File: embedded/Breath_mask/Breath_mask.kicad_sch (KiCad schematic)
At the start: 33 parts, among them IC1 TPS61291DRVR, J1 Conn_01x02_Pin, J2 USB, J4 Conn_ST_STDC14, SW2 SW_Push, SW3 SW_Push, U1 LPS22HBTR, U23 M95256, U4 STM32L052K8Tx

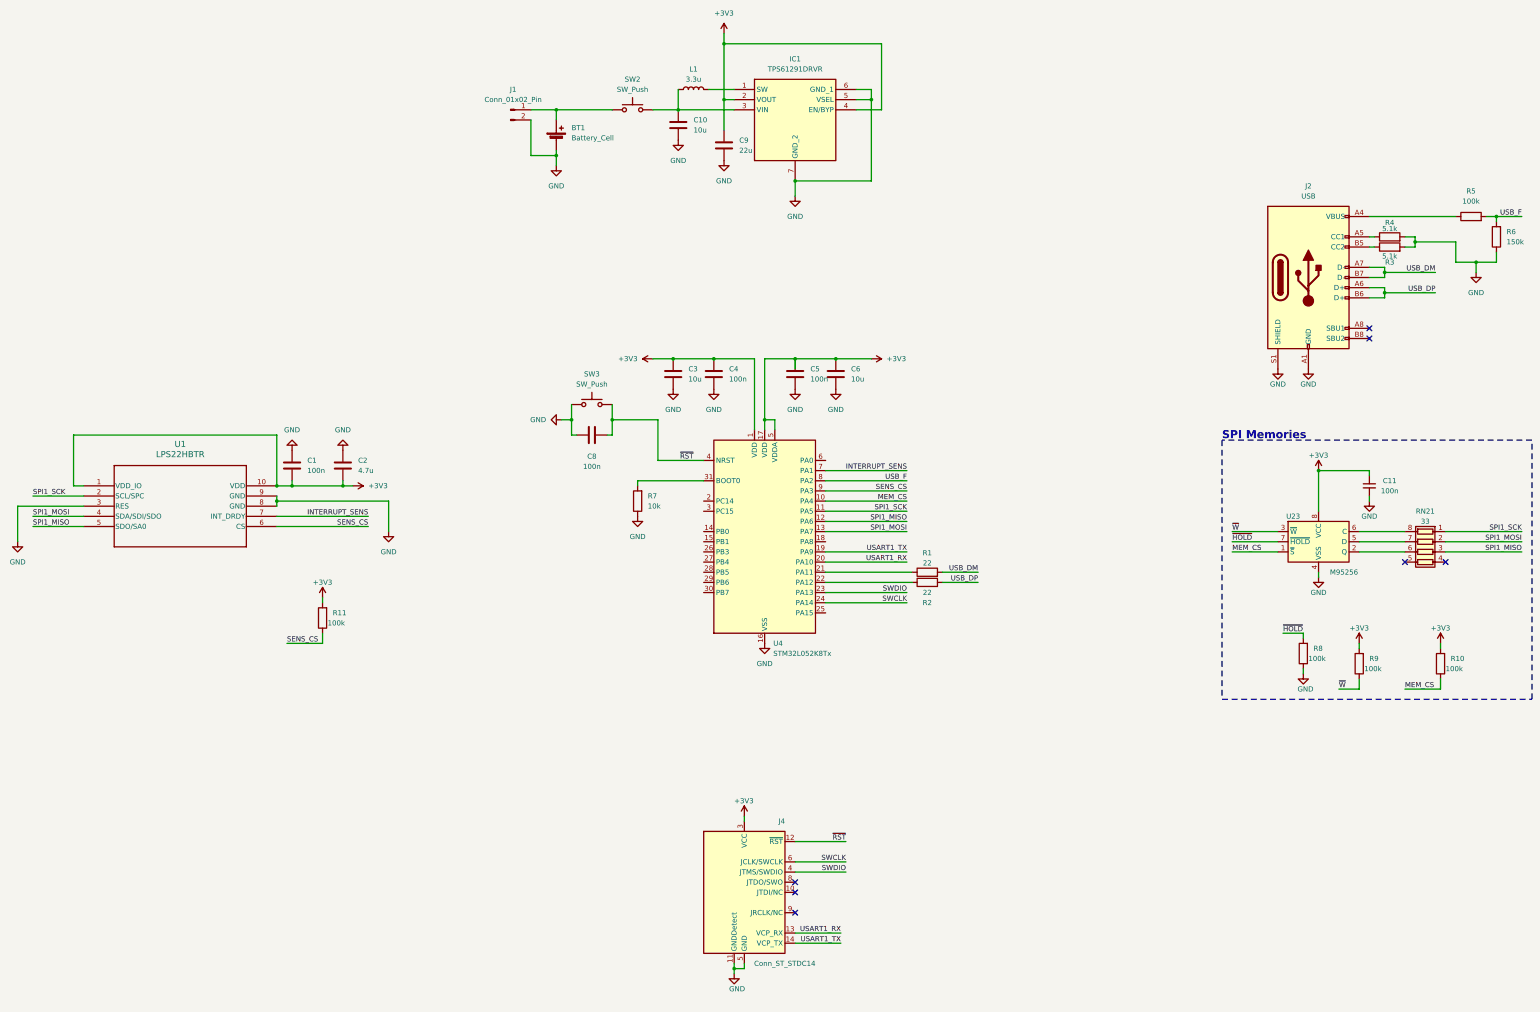
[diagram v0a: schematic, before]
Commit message: inizio sbroglio pcb
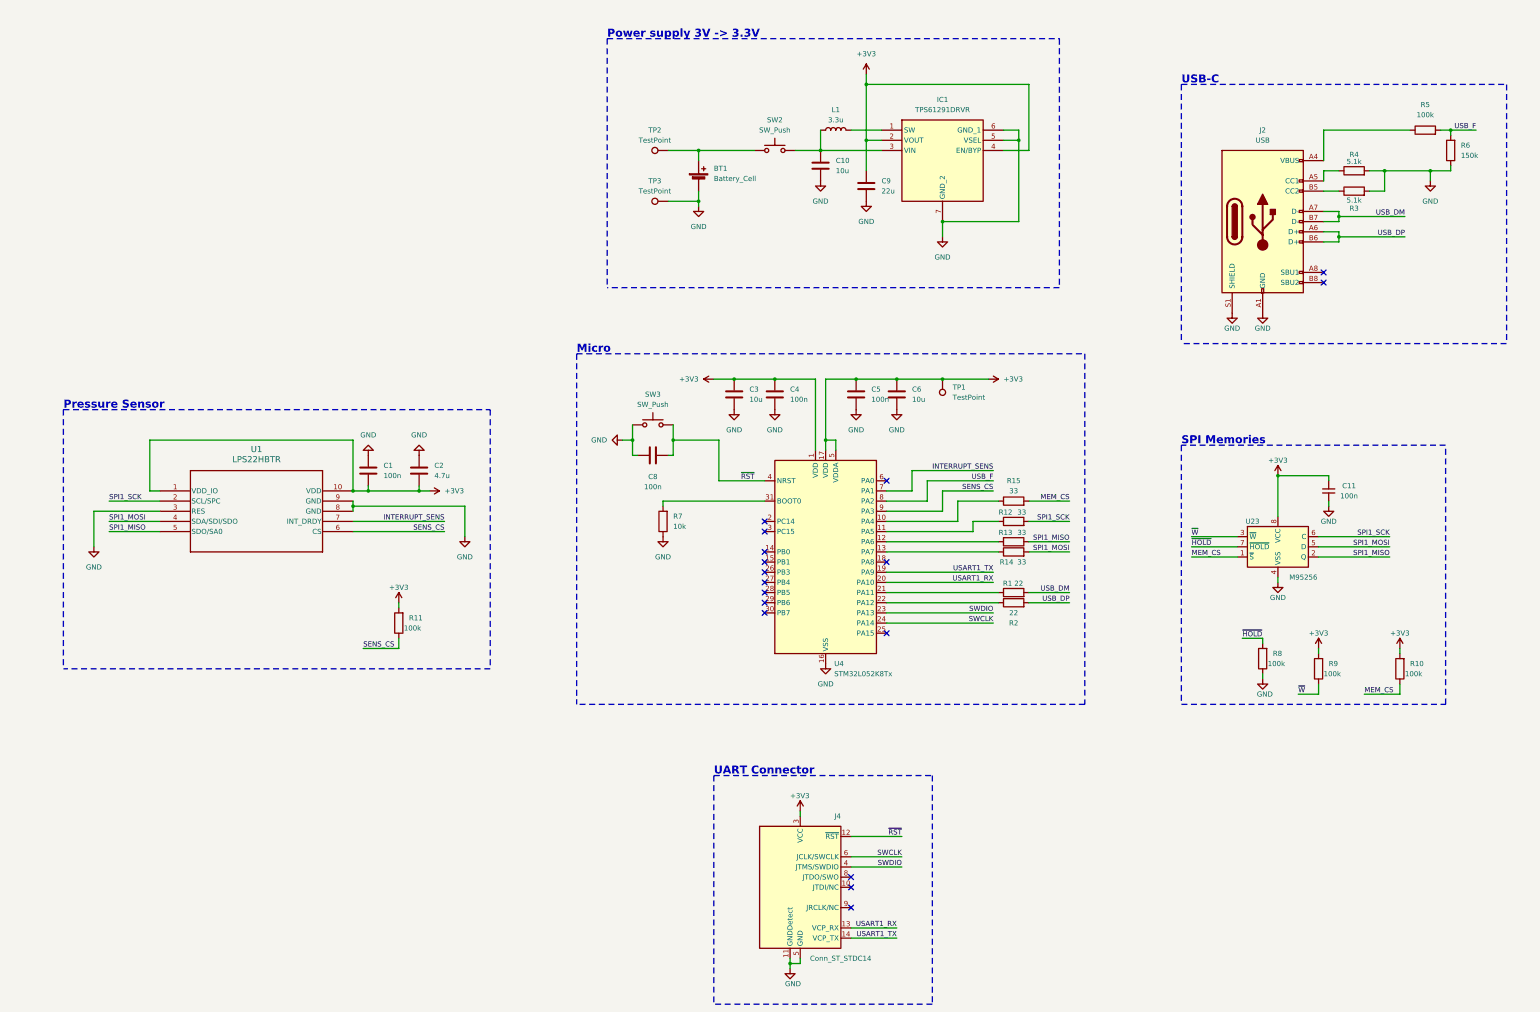
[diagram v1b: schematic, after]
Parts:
- removed J1: Conn_01x02_Pin, symbol Connector:Conn_01x02_Pin
- removed RN21: 33, Resistor_SMD:R_Array_Convex_4x0603, symbol Device:R_Pack04
- added R12, R13, R14, R15: 33, Resistor_SMD:R_0603_1608Metric, symbol Device:R
- added TP1, TP2, TP3: TestPoint, TestPoint:TestPoint_Pad_D1.0mm, symbol Connector:TestPoint
- BT1: footprint (none) -> Battery:BatteryHolder_Keystone_3034_1x20mm
- C1, C2, C4, C5, C8: footprint (none) -> Capacitor_SMD:C_0603_1608Metric
- C10, C3, C6, C9: footprint (none) -> Capacitor_SMD:C_0805_2012Metric
- IC1: footprint SON65P200X200X80-7N -> Package_SON:WSON-6-1EP_2x2mm_P0.65mm_EP1x1.6mm_ThermalVias
- J4: footprint eagle_connectors:SAMTEC_FTSH-107-01-L-DV-K-TR -> impronte_breath_mask:SAMTEC_FTSH-107-01-L-DV-K-TR
- L1: footprint (none) -> Inductor_SMD:L_Coilcraft_LPS3314
- R1, R2, R3, R4, R5, R6, R7: footprint (none) -> Resistor_SMD:R_0603_1608Metric
- SW2: footprint (none) -> Button_Switch_SMD:SW_SPDT_CK_JS102011SAQN
- SW3: footprint (none) -> Button_Switch_SMD:SW_Push_1P1T_XKB_TS-1187A
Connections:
- net +3V3: now also TP1.1
- net GND: now also TP3.1
- net MEM_CS: now also R15.2; no longer U4.10 (PA4)
- net SPI1_MISO: now also U23.2 (Q), R13.1; no longer U4.12 (PA6)
- net SPI1_MOSI: now also U23.5 (D), R14.2; no longer U4.13 (PA7)
- net SPI1_SCK: now also U23.6 (C), R12.2; no longer U4.11 (PA5)
- net at BT1.1 (+), SW2.1: now also TP2.1
- new net: R15.1, U4.10 (PA4)
- new net: R12.1, U4.11 (PA5)
- new net: R13.2, U4.12 (PA6)
- new net: R14.1, U4.13 (PA7)
- no-connect marks 7 -> 17
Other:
- note added: "Micro"
- note added: "Power supply 3V -> 3.3V"
- note added: "Pressure Sensor"
- note added: "UART Connector"
- note added: "USB-C"
- moved on the sheet: C1, C10, C11, C2, C3, C4, C5, C6, C8, C9, IC1, J2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
